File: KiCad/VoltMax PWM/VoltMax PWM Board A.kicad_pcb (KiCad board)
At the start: 2 copper layers, 70 x 20 mm, 32 parts, among them IC1 DS1809Z-010+, IC2 NCV4264-2ST50T3G, J1 BAT-, J2 510-, J3 VIN+, J4 PAD_Fire2, J5 PAD_Fire1, J6 VM-, J7 VM+, Q1 SSM3J334R_LF, Q2 PSMN1R2-25YLC_115, U1 MIC1557YM5_TR

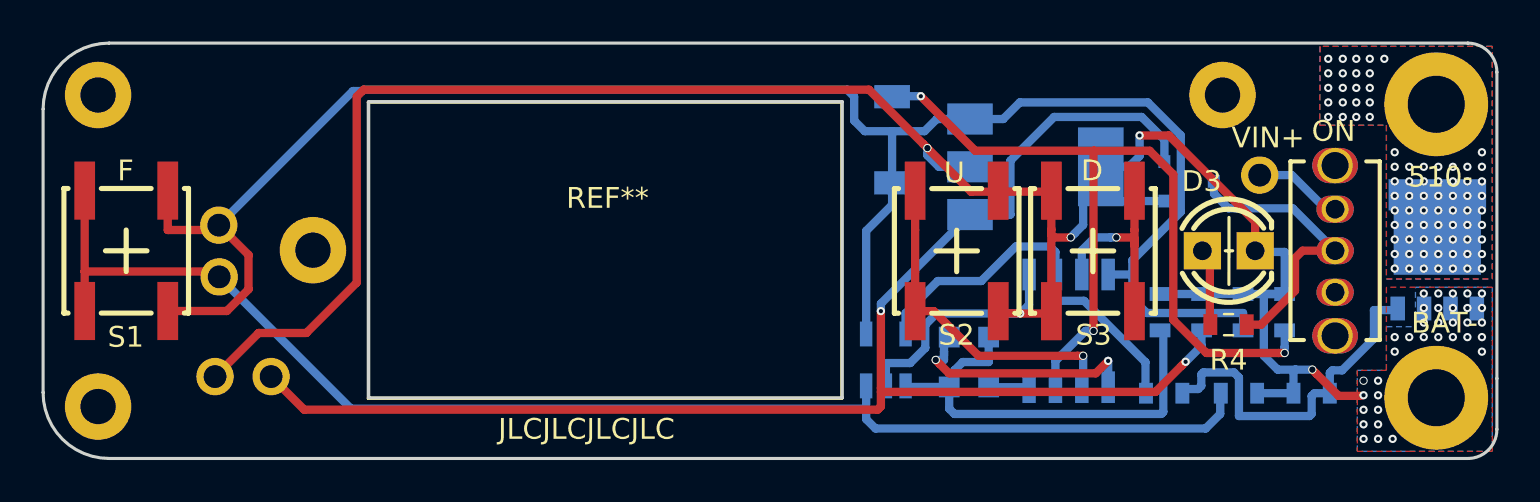
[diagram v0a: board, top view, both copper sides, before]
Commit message: Rename Boards,Add ModMaker/StealthVape box layout
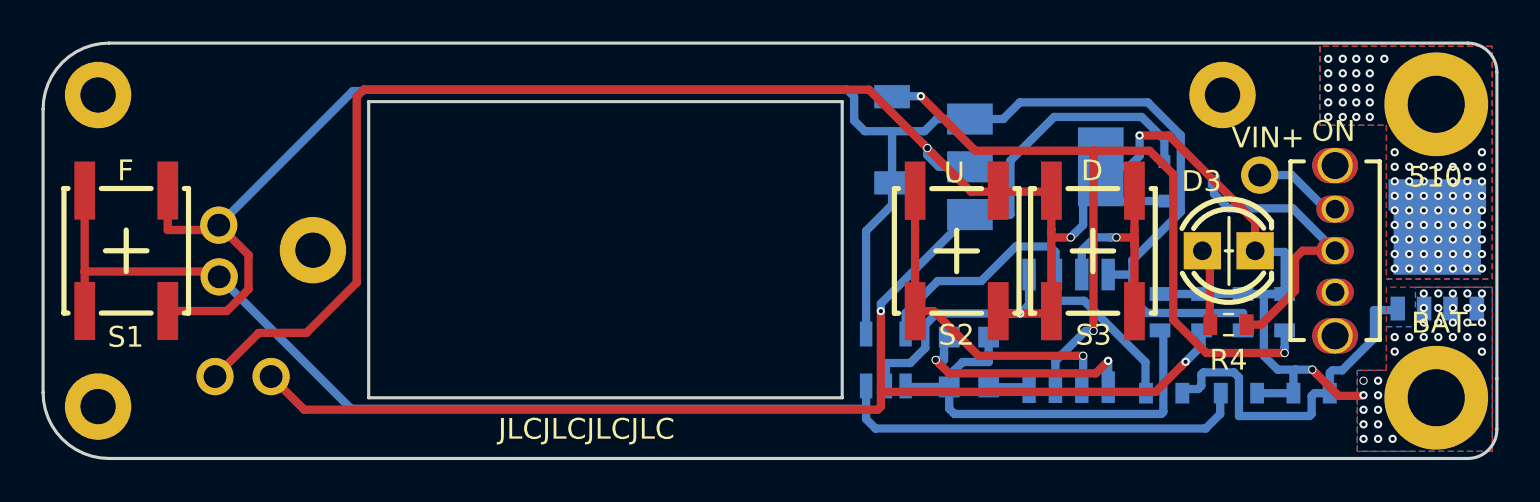
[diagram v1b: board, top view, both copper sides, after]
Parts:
- removed REF**: 0.36_inch_VM, VoltMax PWM:0.36_inch_VM
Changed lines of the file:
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@@
     (tracks 369)
     (zones 0)
-    (modules 32)
+    (modules 31)
     (nets 20)
   )
@@
       (drillshape 0)
       (scaleselection 1)
-      (outputdirectory "Gerbers-ATI/"))
+      (outputdirectory "Gerbers-Board A/"))
   )
   (net 0 "")
@@
       (rotate (xyz -90 0 0))
     )
-  )
-  (module "VoltMax PWM:0.36_inch_VM" (layer F.Cu)
-    (at 141.7 100.3)
-    (fp_text reference REF** (at 0 -2.69) (layer F.SilkS)
-      (effects (font (size 1 1) (thickness 0.15)))
-    )
-    (fp_text value 0.36_inch_VM (at 0 -0.73) (layer F.Fab) hide
-      (effects (font (size 1 1) (thickness 0.15)))
-    )
-    (fp_line (start 11.2781 -7.3084) (end -11.5219 -7.3084) (layer F.SilkS) (width 0.15))
-    (fp_line (start -11.5219 -7.3084) (end -11.5219 6.9516) (layer F.SilkS) (width 0.15))
-    (fp_line (start -11.5219 6.9516) (end 11.2781 6.9516) (layer F.SilkS) (width 0.15))
-    (fp_line (start 11.2781 6.9516) (end 11.2781 -7.3084) (layer F.SilkS) (width 0.15))
-    (model "${KIPRJMOD}/VoltMax PWM.pretty/XDxx09x3.step"
-      (offset (xyz -0.1 0.15 4.45))
-      (scale (xyz 1.018 1 1.022))
-      (rotate (xyz -90 0 0))
-    )
